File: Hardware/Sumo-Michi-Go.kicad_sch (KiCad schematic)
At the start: 17 parts, among them J1 ENTRADA, J10 ENTRADA, J11 Conn_01x10, J2 Conn_01x04, J3 Conn_01x09_Pin, J4 SENSOR_INFRAROJO_1, J5 ULTRASONIDO_1, J6 ULTRASONIDO_2, J7 SENSOR_INFRAROJO_2, J8 SENSOR_INFRAROJO_3, J9 ENTRADA, SW1 SWITCH_ON_OFF, SW2 SW_DE_INICIO_ROBOT

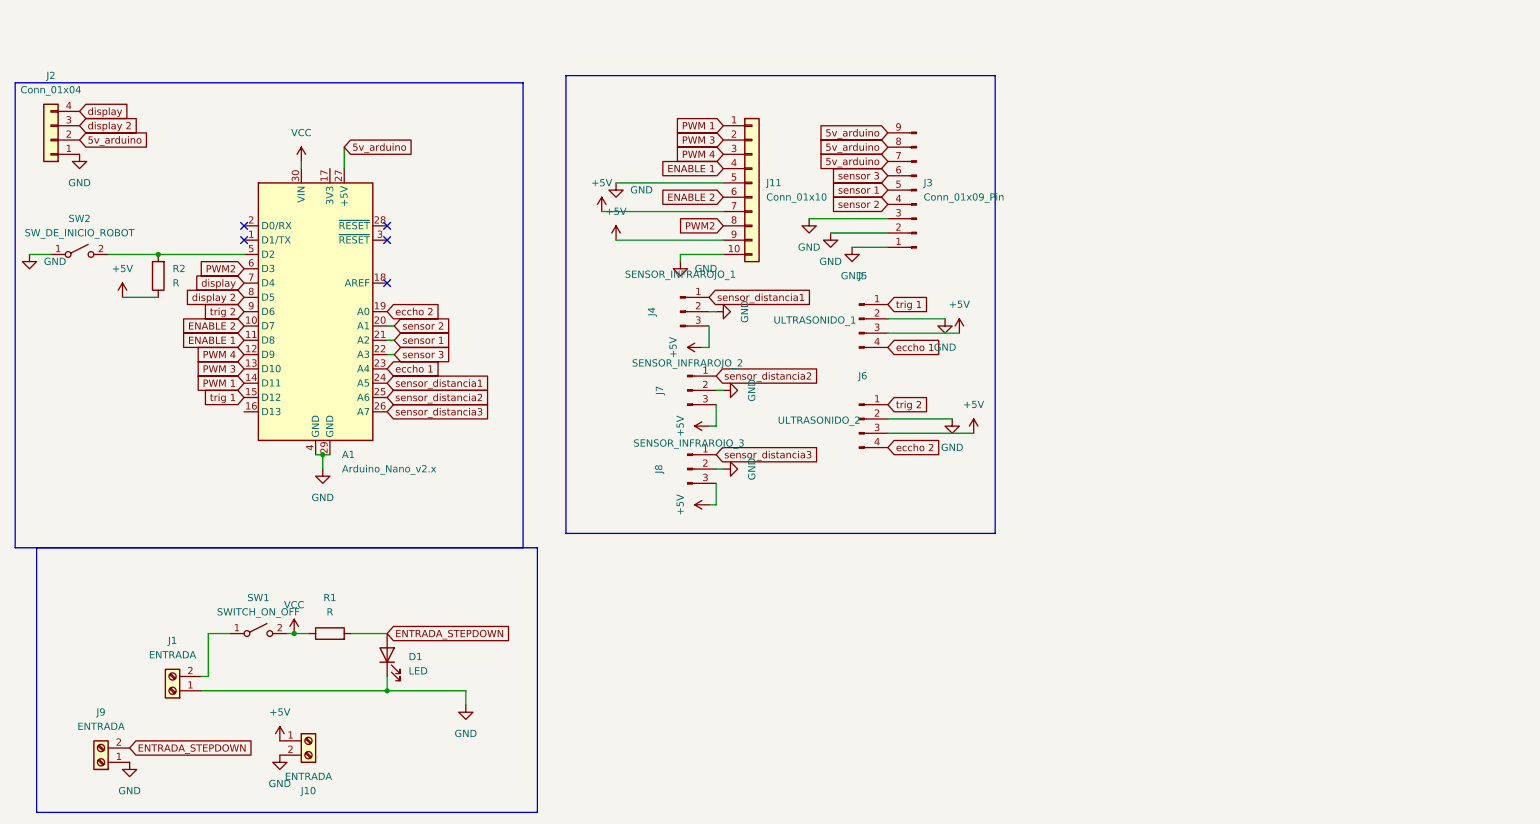
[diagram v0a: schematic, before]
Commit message: PCB nuevo
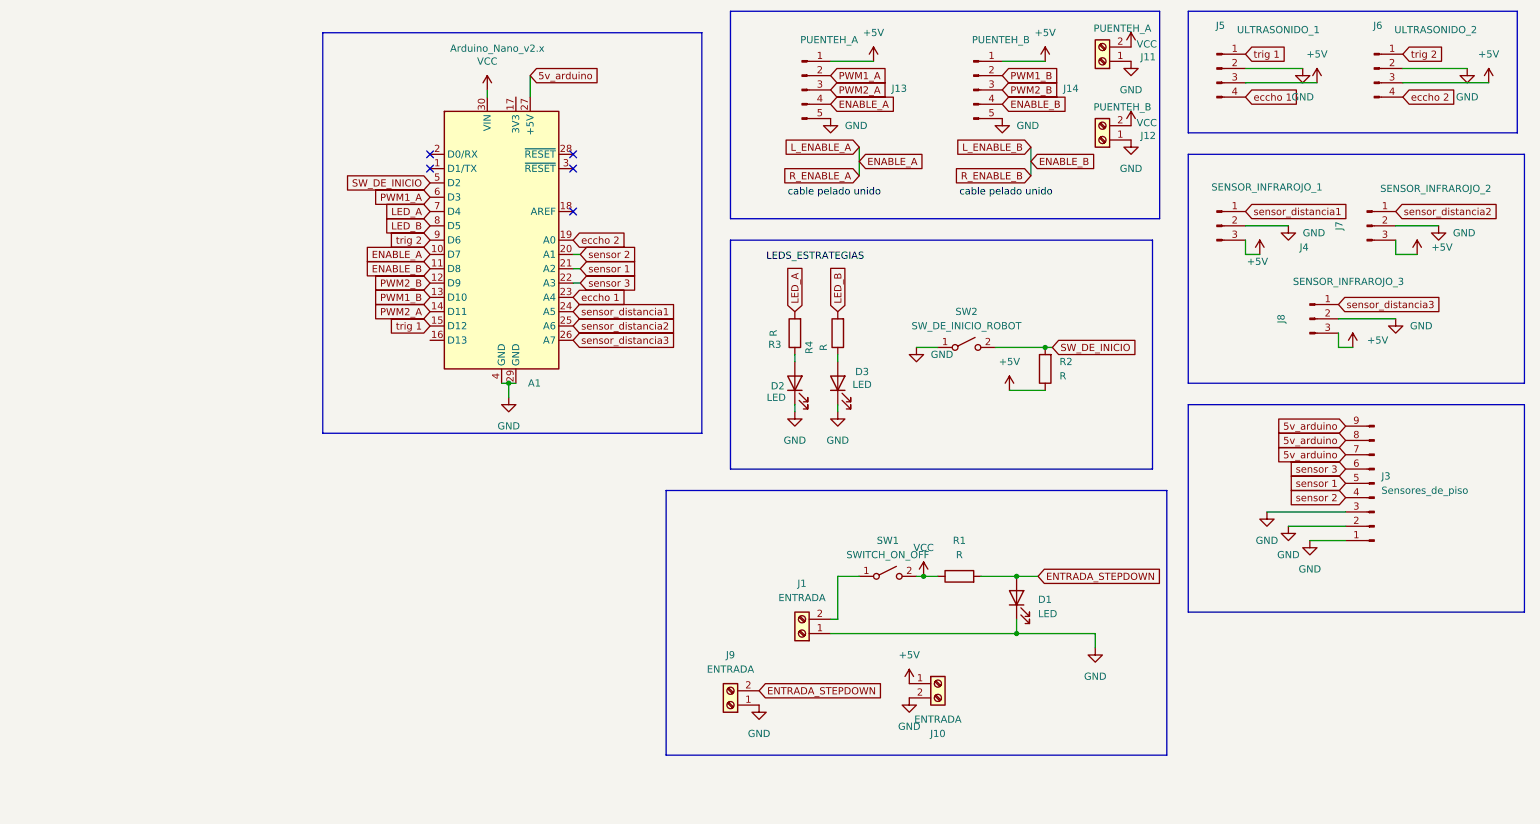
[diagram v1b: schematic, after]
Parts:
- removed J11: Conn_01x10, Connector_PinHeader_2.54mm:PinHeader_1x10_P2.54mm_Vertical, symbol Connector_Generic:Conn_01x10
- removed J2: Conn_01x04, Connector_PinHeader_2.54mm:PinHeader_1x04_P2.54mm_Vertical, symbol Connector_Generic:Conn_01x04
- added D2, D3: LED, LED_THT:LED_D5.0mm_Clear, symbol Device:LED
- added J11: PUENTEH_A, TerminalBlock:TerminalBlock_Altech_AK300-2_P5.00mm, symbol Connector:Screw_Terminal_01x02
- added J12: PUENTEH_B, TerminalBlock:TerminalBlock_Altech_AK300-2_P5.00mm, symbol Connector:Screw_Terminal_01x02
- added J13: PUENTEH_A, Connector_PinSocket_2.54mm:PinSocket_1x05_P2.54mm_Vertical, symbol Connector:Conn_01x05_Pin
- added J14: PUENTEH_B, Connector_PinSocket_2.54mm:PinSocket_1x05_P2.54mm_Vertical, symbol Connector:Conn_01x05_Pin
- added R3, R4: R, Resistor_SMD:R_0805_2012Metric, symbol Device:R
- D1: footprint Inductor_SMD:L_0805_2012Metric_Pad1.15x1.40mm_HandSolder -> LED_THT:LED_D5.0mm_Clear
- J3: value Conn_01x09_Pin -> Sensores_de_piso
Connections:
- net +5V: now also J13.1 (Pin_1), J14.1 (Pin_1)
- net GND: now also D2.1 (K), D3.1 (K), J11.1 (Pin_1), J12.1 (Pin_1), J13.5 (Pin_5), J14.5 (Pin_5)
- net VCC: now also J11.2 (Pin_2), J12.2 (Pin_2)
- net SW_DE_INICIO: now reaches A1.5 (D2), R2.2, SW2.2 (B)
- net ENABLE 1 renamed ENABLE_B
- net ENABLE_B: now also J14.4 (Pin_4)
- net ENABLE 2 renamed ENABLE_A
- net ENABLE_A: now also J13.4 (Pin_4)
- net PWM 1 renamed PWM2_A
- net PWM2_A: now also J13.3 (Pin_3)
- net PWM 3 renamed PWM1_B
- net PWM1_B: now also J14.2 (Pin_2)
- net PWM 4 renamed PWM2_B
- net PWM2_B: now also J14.3 (Pin_3)
- net PWM2 renamed PWM1_A
- net PWM1_A: now also J13.2 (Pin_2)
- net display renamed LED_A
- net LED_A: now also R3.2
- net display 2 renamed LED_B
- net LED_B: now also R4.2
- new net: D2.2 (A), R3.1
- new net: D3.2 (A), R4.1
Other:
- moved on the sheet: A1, D1, J1, J10, J3, J4, J5, J6, J7, J8, J9, R1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
